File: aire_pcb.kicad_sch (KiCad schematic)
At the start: 56 parts, among them J1 Conn_01x02_Male, J2 Screw_Terminal_01x02, J3 Screw_Terminal_01x03, J4 Conn_01x04_Male, J5 Conn_02x04_Top_Bottom, K1 JRC-21F_4100, K2 JRC-21F_4100, K3 JRC-21F_4100, Q1 2N3904, Q2 2N3904, Q3 2N3904, SW1 SW_Push, SW2 SW_Push, U1 NCP1117-3.3_SOT223, U2 HLK-2M05, U3 SHT40, U4 ESP8266-12E{slash}ESP-12E

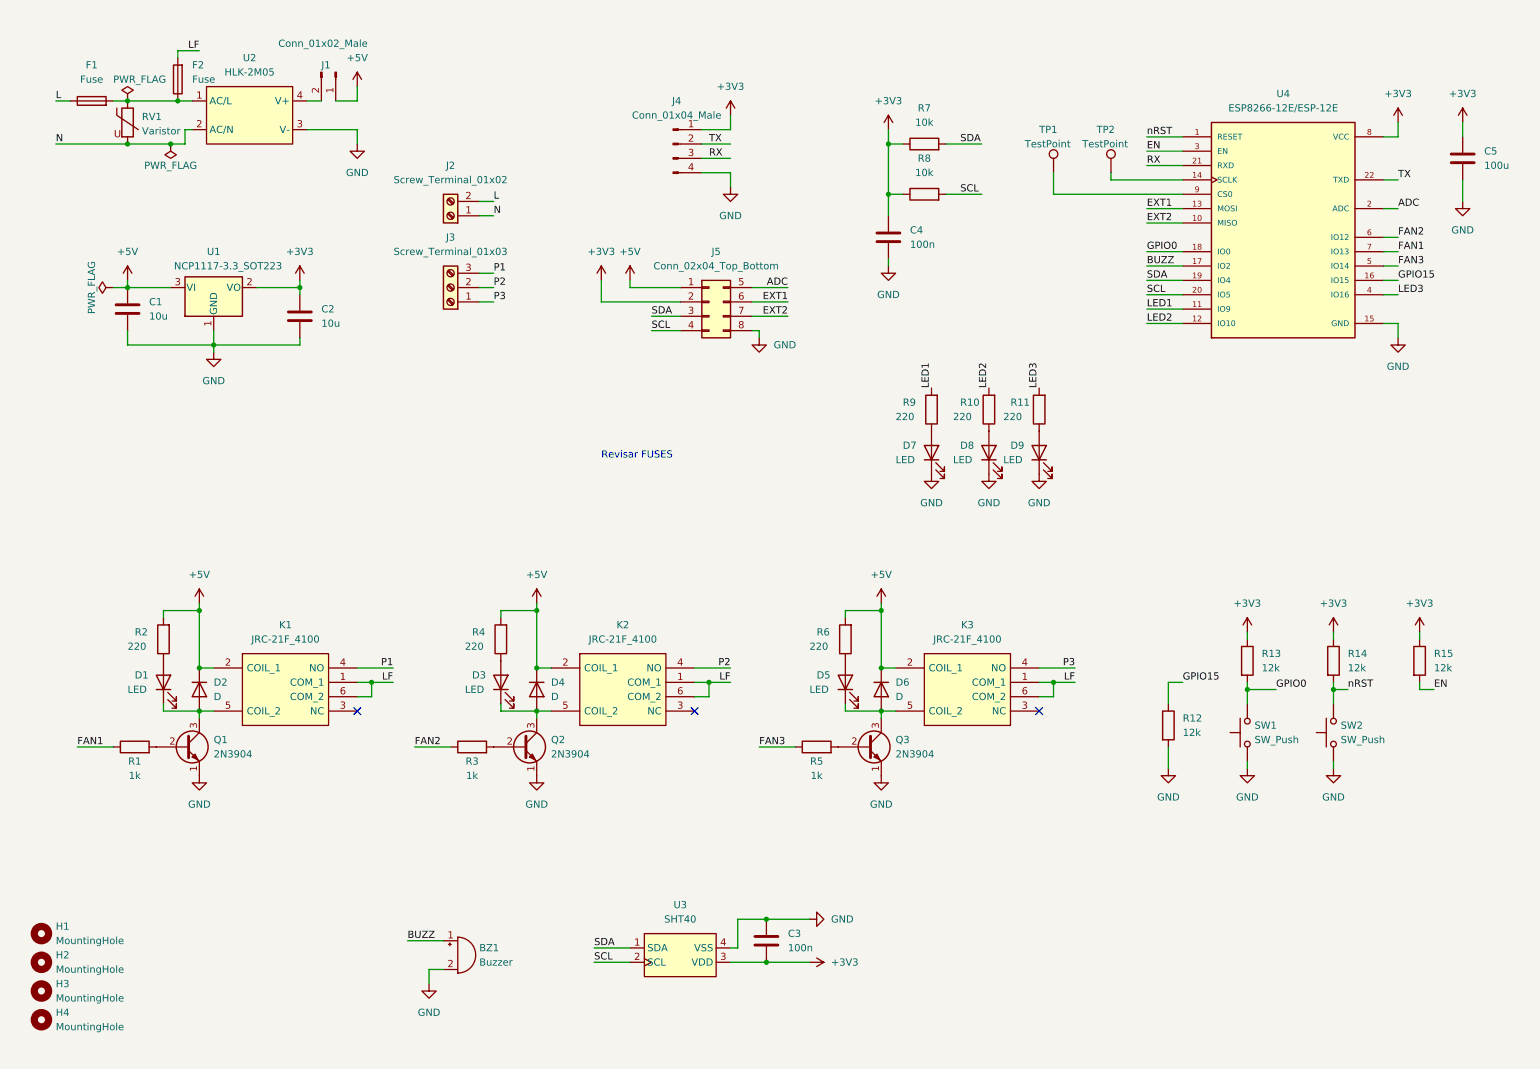
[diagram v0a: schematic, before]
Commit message: Minor redesign
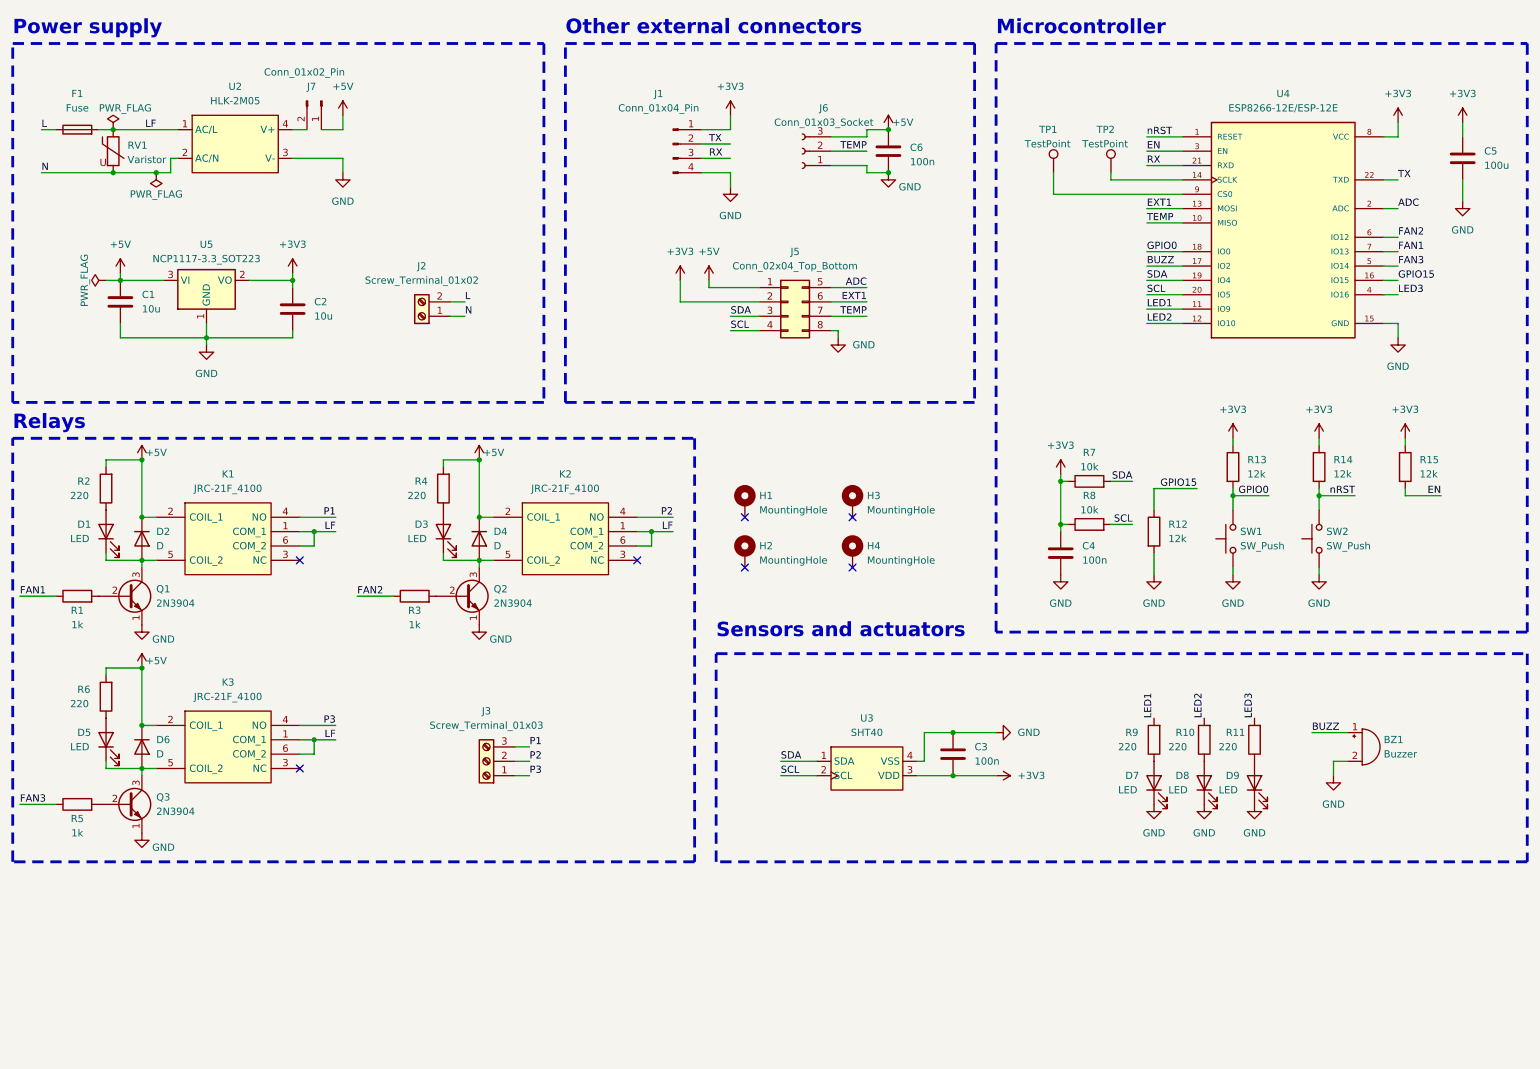
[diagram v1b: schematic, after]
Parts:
- removed F2: Fuse, guille_3rdparty:Fuse_2512_6332Metric, symbol Device:Fuse
- removed J1: Conn_01x02_Male, Connector_PinHeader_2.54mm:PinHeader_1x02_P2.54mm_Vertical, symbol Connector:Conn_01x02_Male
- removed J4: Conn_01x04_Male, Connector_PinHeader_2.54mm:PinHeader_1x04_P2.54mm_Vertical, symbol Connector:Conn_01x04_Male
- removed U1: NCP1117-3.3_SOT223, Package_TO_SOT_SMD:SOT-223-3_TabPin2, symbol Regulator_Linear:NCP1117-3.3_SOT223
- added C6: 100n, Capacitor_SMD:C_0402_1005Metric, symbol Device:C
- added J1: Conn_01x04_Pin, Connector_PinHeader_2.54mm:PinHeader_1x04_P2.54mm_Vertical, symbol Connector:Conn_01x04_Pin
- added J6: Conn_01x03_Socket, Connector_PinSocket_2.54mm:PinSocket_1x03_P2.54mm_Vertical, symbol Connector:Conn_01x03_Socket
- added J7: Conn_01x02_Pin, Connector_PinHeader_2.54mm:PinHeader_1x02_P2.54mm_Vertical, symbol Connector:Conn_01x02_Pin
- added U5: NCP1117-3.3_SOT223, Package_TO_SOT_SMD:SOT-223-3_TabPin2, symbol Regulator_Linear:NCP1117-3.3_SOT223
- H1, H2, H3, H4: footprint MountingHole:MountingHole_3.2mm_M3_DIN965 -> MountingHole:MountingHole_3.2mm_M3_Pad_TopBottom; symbol Mechanical:MountingHole -> Mechanical:MountingHole_Pad
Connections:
- net +3V3: now also J1.1 (Pin_1), U5.2 (VO)
- net +5V: now also C6.1, J6.3 (Pin_3), J7.1 (Pin_1), U5.3 (VI)
- net GND: now also C6.2, J1.4 (Pin_4), J6.1 (Pin_1), U5.1 (GND)
- net LF: now also F1.2, RV1.1, U2.1 (AC/L)
- net RX: now also J1.3 (Pin_3)
- net TX: now also J1.2 (Pin_2)
- net at U2.4 (V+): now also J7.2 (Pin_2)
- net EXT2 renamed TEMP
- net TEMP: now also J6.2 (Pin_2)
- no-connect marks 3 -> 7
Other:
- note added: "Microcontroller"
- note added: "Other external connectors"
- note added: "Power supply"
- note added: "Relays"
- note added: "Sensors and actuators"
- note removed: "Revisar FUSES"
- moved on the sheet: BZ1, C1, C2, C3, C4, D1, D2, D3, D4, D5, D6, D7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

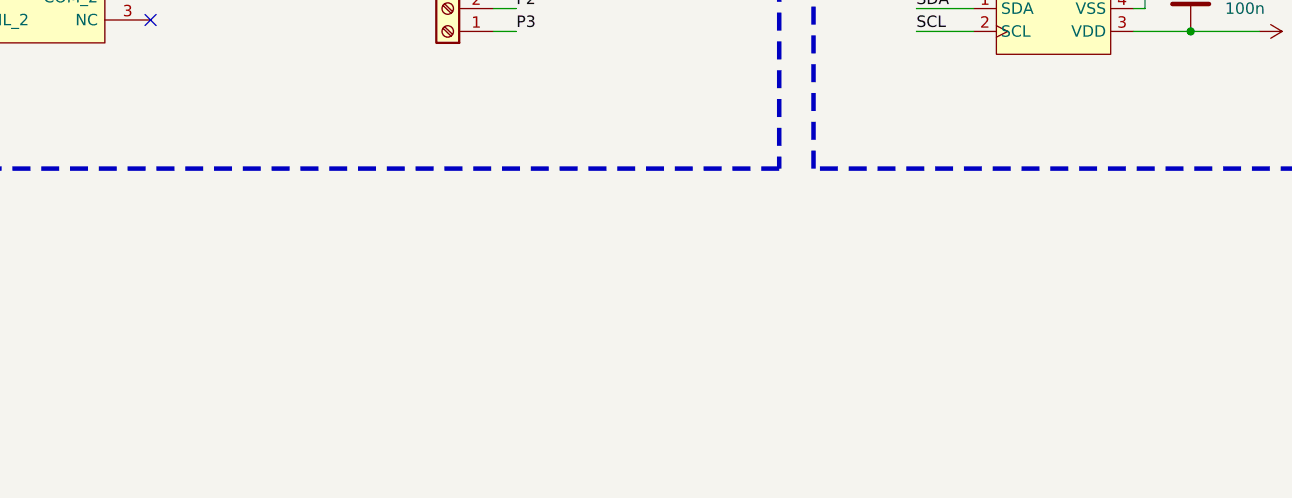
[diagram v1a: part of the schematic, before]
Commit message: PCB changes
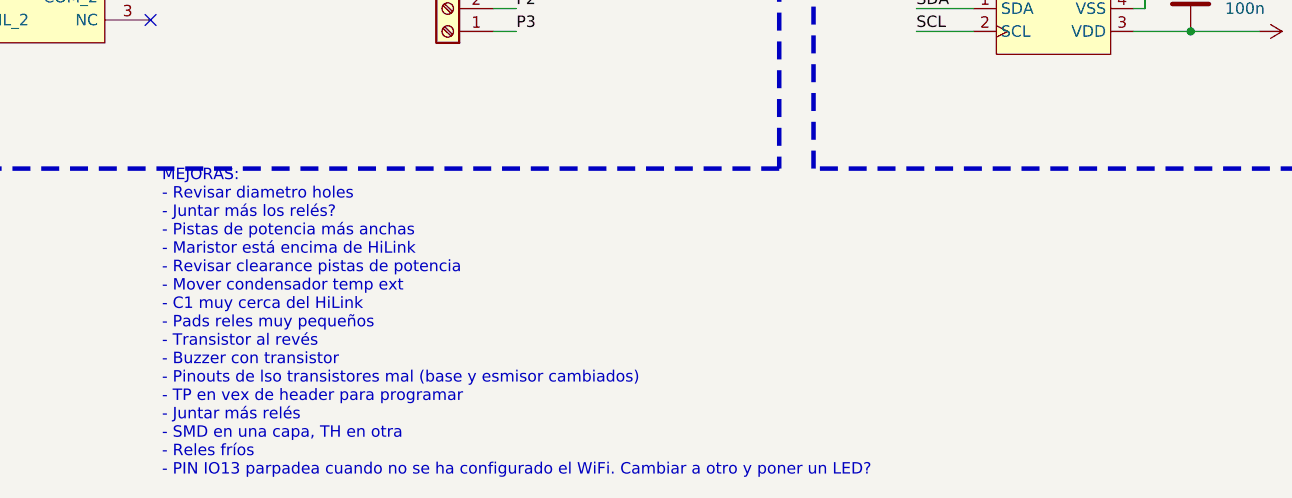
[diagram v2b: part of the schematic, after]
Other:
- note added: "MEJORAS: - Revisar diametro holes - Juntar más los relés? - Pistas de potencia más anchas - Maristor está encima de HiLink - Revisar clearance pistas de potencia - Mover condensador temp ext - C1 muy cerca del HiLink - Pads reles muy pequeños - Transistor al revés - Buzzer con transistor - Pinouts de lso transistores mal (base y esmisor cambiados) - TP en vex de header para programar - Juntar más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"
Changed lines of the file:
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@@
     (effects (font (size 2.54 2.54) (thickness 0.508) bold) (justify left bottom))
+  )
+  (text "MEJORAS:\n- Revisar diametro holes\n- Juntar más los relés?\n- Pistas de potencia más anchas\n- Maristor está encima de HiLink\n- Revisar clearance pistas de potencia\n- Mover condensador temp ext\n- C1 muy cerca del HiLink\n- Pads reles muy pequeños\n- Transistor al revés\n- Buzzer con transistor\n- Pinouts de lso transistores mal (base y esmisor cambiados)\n- TP en vex de header para programar\n- Juntar más relés\n- SMD en una capa, TH en otra\n- Reles fríos\n- PIN IO13 parpadea cuando no se ha configurado el WiFi. Cambiar a otro y poner un LED?"
+    (at 67.31 196.85 0)
+    (effects (font (size 1.27 1.27)) (justify left bottom))
   )
   (text "Sensors and actuators" (at 139.7 123.19 0)
